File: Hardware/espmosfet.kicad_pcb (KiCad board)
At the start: 2 copper layers, 32 x 42 mm, 59 parts, among them J1 USB_B_Micro, J2 Conn_01x04_Male, J3 USB_A, J4 Conn_01x04_Male, J5 Conn_01x02_Male, J6 Conn_01x02_Male, J7 Conn_01x03_Male, P1 USB_C_Receptacle_USB2.0, P2 USB_C_Receptacle_USB2.0, Q1 AO3400A, Q2 AO3400A, SW1 SW_Push, U1 TPS2514A, U2 ESP-12F, U3 LM1117-3.3, U4 INA226, U5 SN74LVC1T45DBV, U6 LMZM23601V5

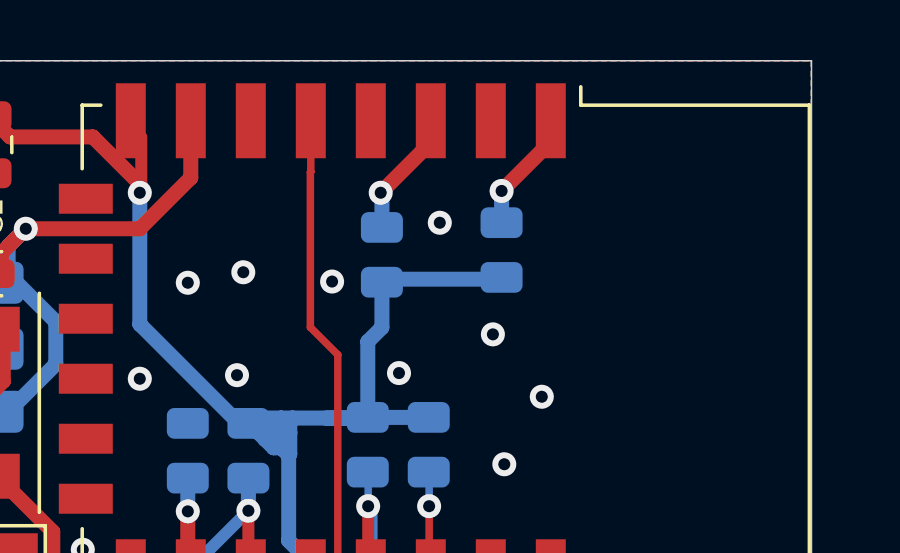
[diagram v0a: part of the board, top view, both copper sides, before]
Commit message: Update espmosfet.kicad_pcb
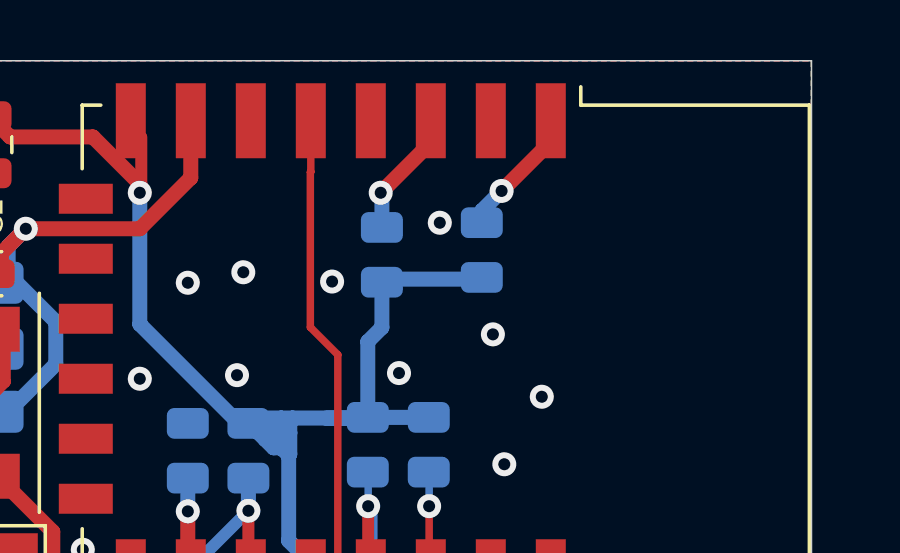
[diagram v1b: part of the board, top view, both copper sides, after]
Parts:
- added G***: LOGO, LOGO, B.Cu at (119.8, 105.2)
- moved R2 0.66 mm to (114.0, 106.3)
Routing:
- net +3V3: track 106.7 -> 106.0 mm
